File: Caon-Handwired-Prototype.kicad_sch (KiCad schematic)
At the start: 179 parts, among them J1 OLED_128x32, SW30 EC11 ENCODER 1, SW45 EC11 ENCODER 1, U1 74HC595, U2 74HC595, U3 SuperMini nRF52840

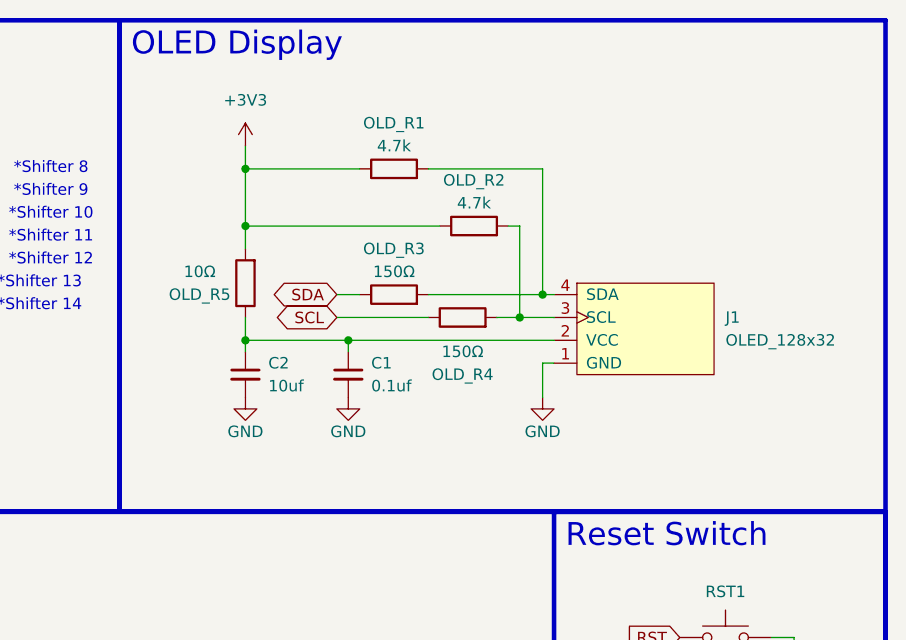
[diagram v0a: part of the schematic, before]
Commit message: Readibility
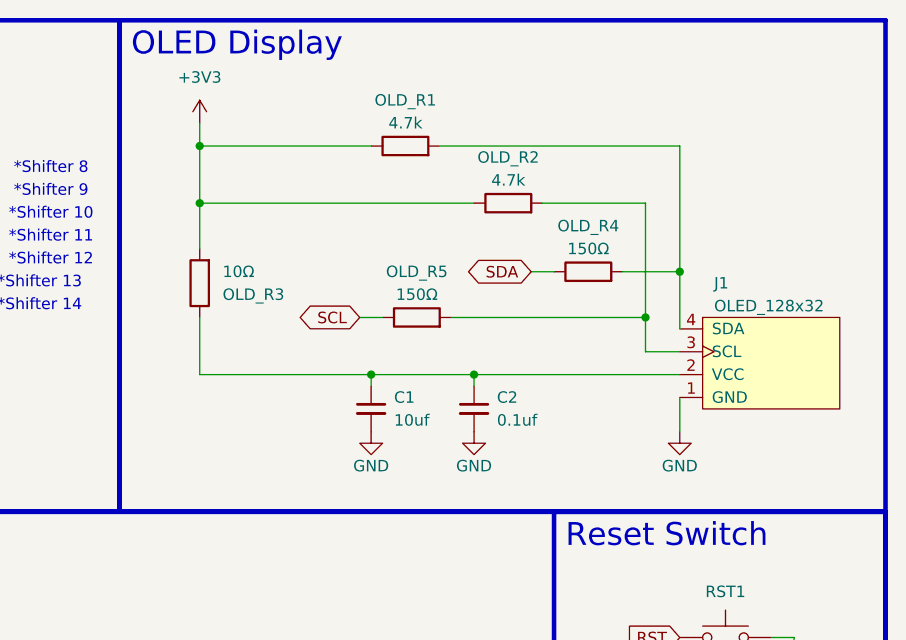
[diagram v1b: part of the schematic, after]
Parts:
- renumbered C2 to C1, C1 to C2, OLD_R5 to OLD_R3, OLD_R3 to OLD_R4, OLD_R4 to OLD_R5
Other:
- moved on the sheet: C1, C2, J1, OLD_R1, OLD_R2, OLD_R3, OLD_R4, OLD_R5
